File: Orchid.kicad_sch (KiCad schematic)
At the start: 130 parts, among them J1 Battery_L, J2 Battery_R, SW1 SW_DPDT_x2, SW2 SW_DPDT_x2, U1 nice_nano, U2 nice_nano

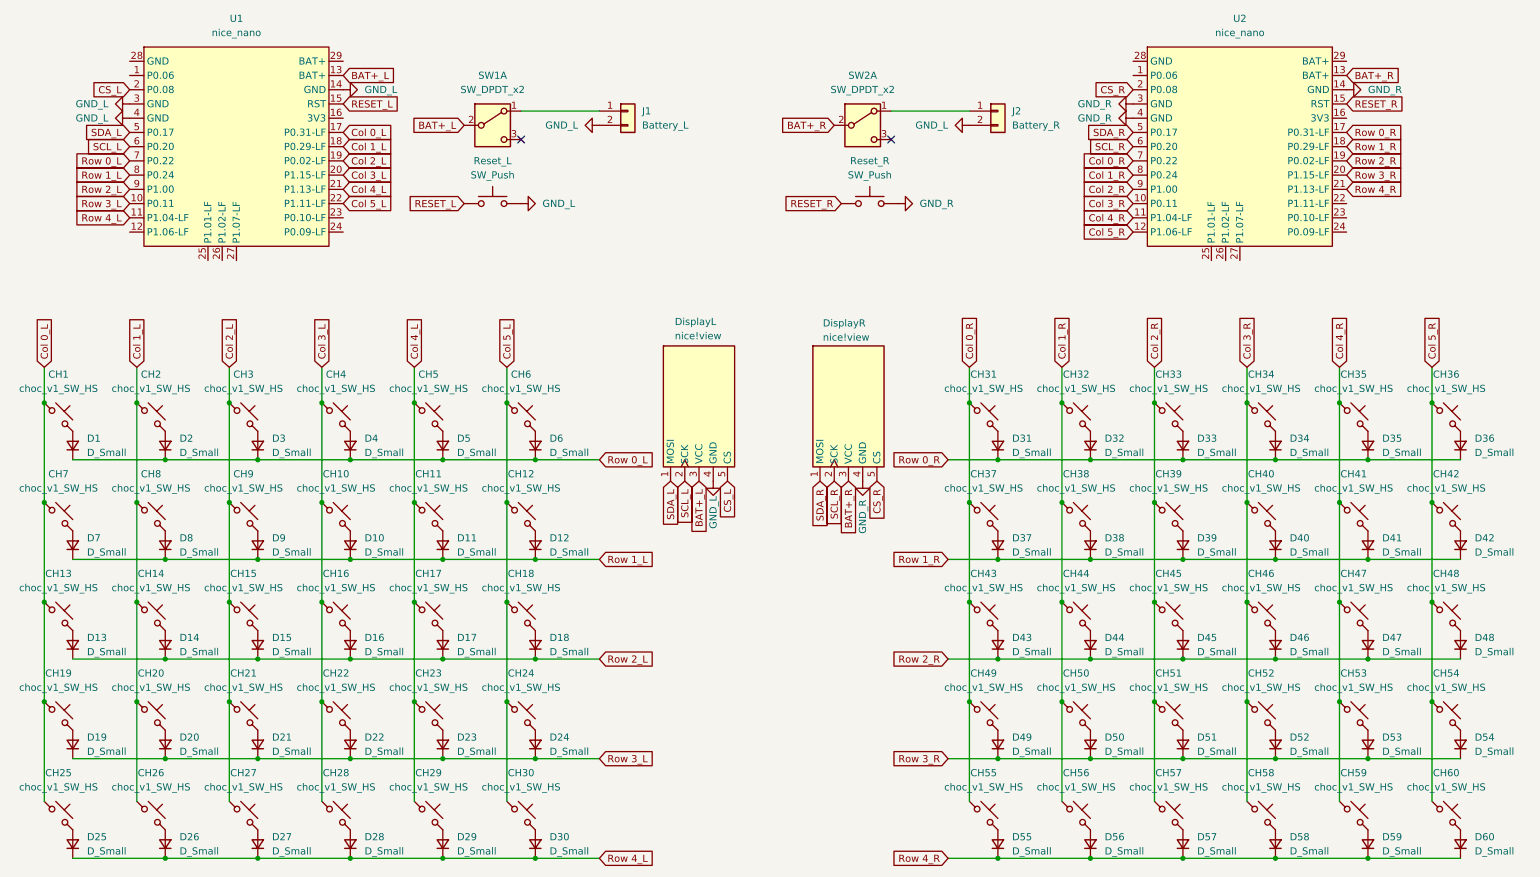
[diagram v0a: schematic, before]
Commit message: vcc.
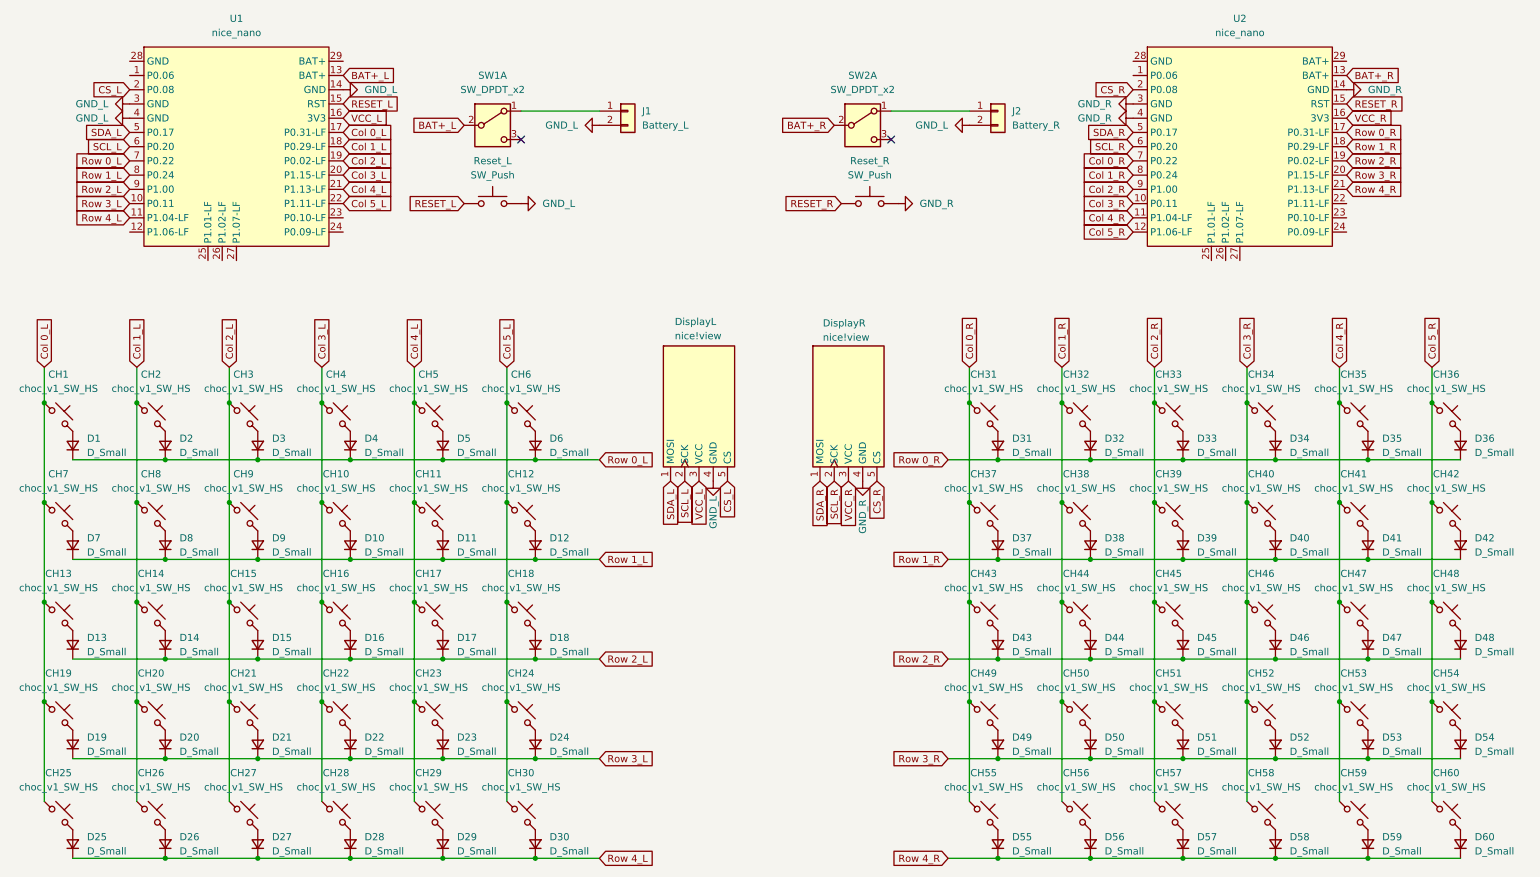
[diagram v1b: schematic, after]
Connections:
- net BAT+_L: no longer DisplayL.3 (VCC)
- net BAT+_R: no longer DisplayR.3 (VCC)
- net VCC_R: now reaches U2.16 (3V3)
- net VCC_R: now also DisplayR.3 (VCC)
- net VCC_L: now reaches U1.16 (3V3)
- net VCC_L: now also DisplayL.3 (VCC)
